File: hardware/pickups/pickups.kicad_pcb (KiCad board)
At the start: 2 copper layers, 40.5 x 45 mm, 6 parts

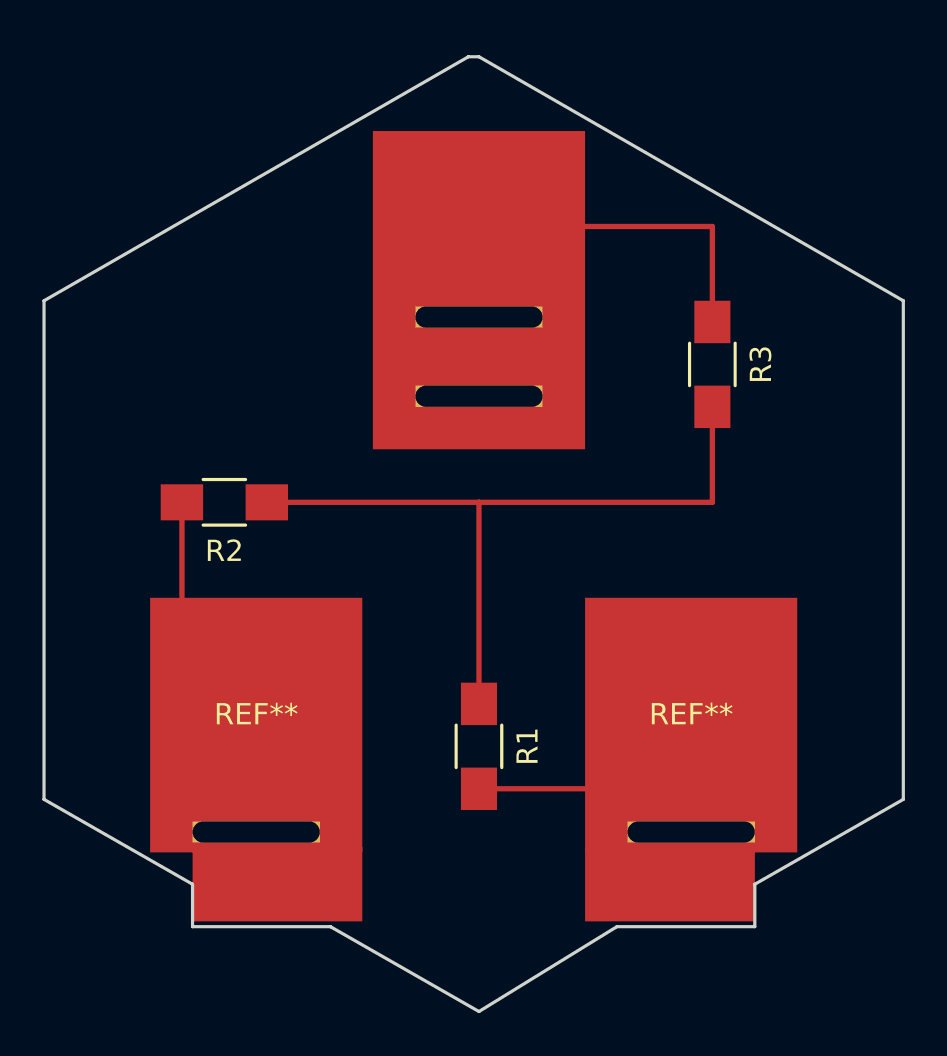
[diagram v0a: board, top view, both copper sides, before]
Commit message: Update pickups pcb
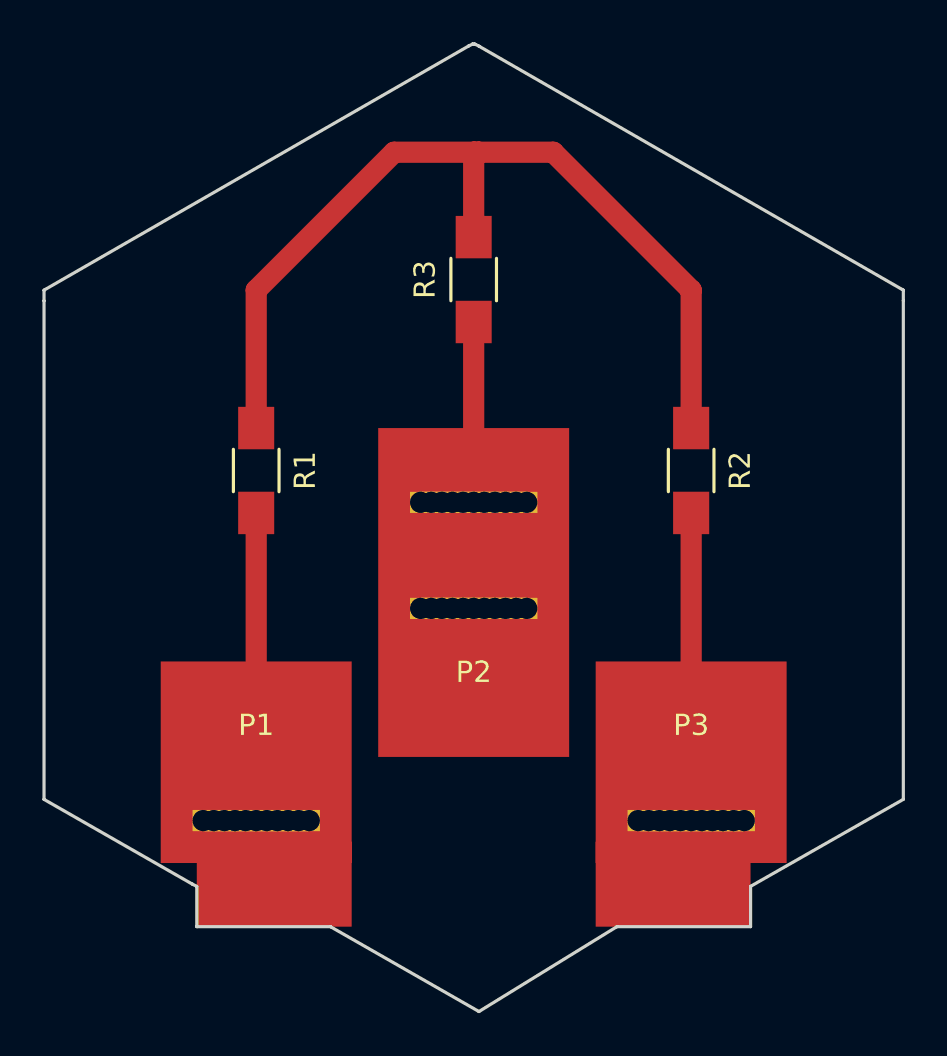
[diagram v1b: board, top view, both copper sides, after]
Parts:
- removed Out: Out, moonbeaminteractive:pickup_contact
- removed REF**: VCC, pickup_contact_bottom_right
- removed REF**: GND, moonbeaminteractive:pickup_contact_bottom_left
- added P1: VCC, pickup_contact_bottom_left, F.Cu at (97.5, 95.5)
- added P2: OUT, pickup_contact, F.Cu at (107.8, 87.0)
- added P3: GND, pickup_contact_bottom_right, F.Cu at (118.0, 95.5)
- moved R2 22.1 mm to (118.0, 80.5), turned to 270 degrees
- moved R1 16.7 mm to (97.5, 80.5)
- moved R3 11.9 mm to (107.8, 71.5), turned to 90 degrees
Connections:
- R1 pad 2: GND -> Net-(P1-Pad1)
- R2 pad 2: VCC -> Net-(P3-Pad1)
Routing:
- net Net-(P3-Pad1): track 0.00 -> 8.75 mm
- net Net-(P1-Pad1): track 0.00 -> 8.75 mm
- net Net-(R1-Pad1): track 35.0 -> 43.1 mm
- net Net-(P2-Pad1): track 12.5 -> 6.25 mm
- net VCC: track 6.00 -> 0.00 mm
- net GND: track 5.50 -> 0.00 mm
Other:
- board size 40.5 x 45 mm -> 40.5 x 45.6 mm
- net class Default: clearance 0.2 -> 0.8; trace_width 0.25 -> 1
- net class Pickup added: clearance 0.8, trace_width 1, via_dia 0.6, via_drill 0.4
- rule trace_clearance: 0.2 -> 0.8
